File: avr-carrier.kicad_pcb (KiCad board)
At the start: 2 copper layers, 71.5 x 71.5 mm, 0 parts

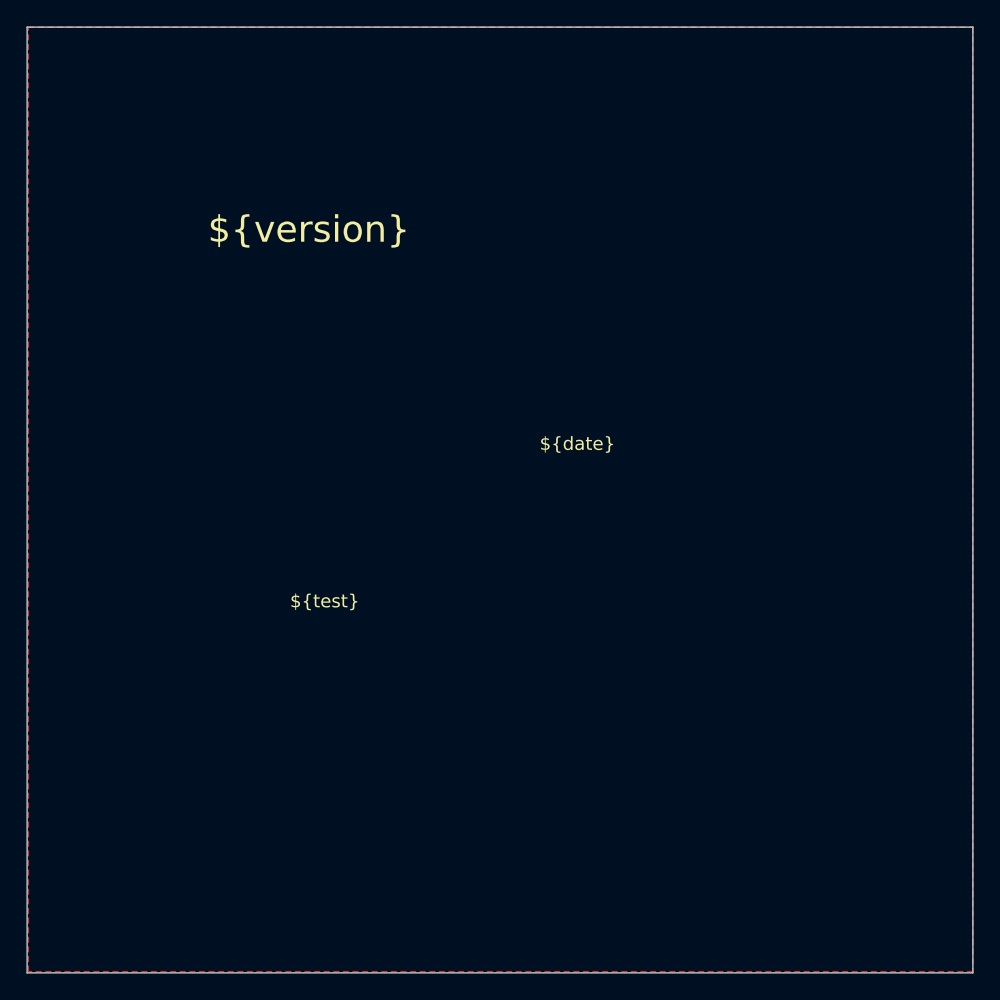
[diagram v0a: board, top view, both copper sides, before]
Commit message: init
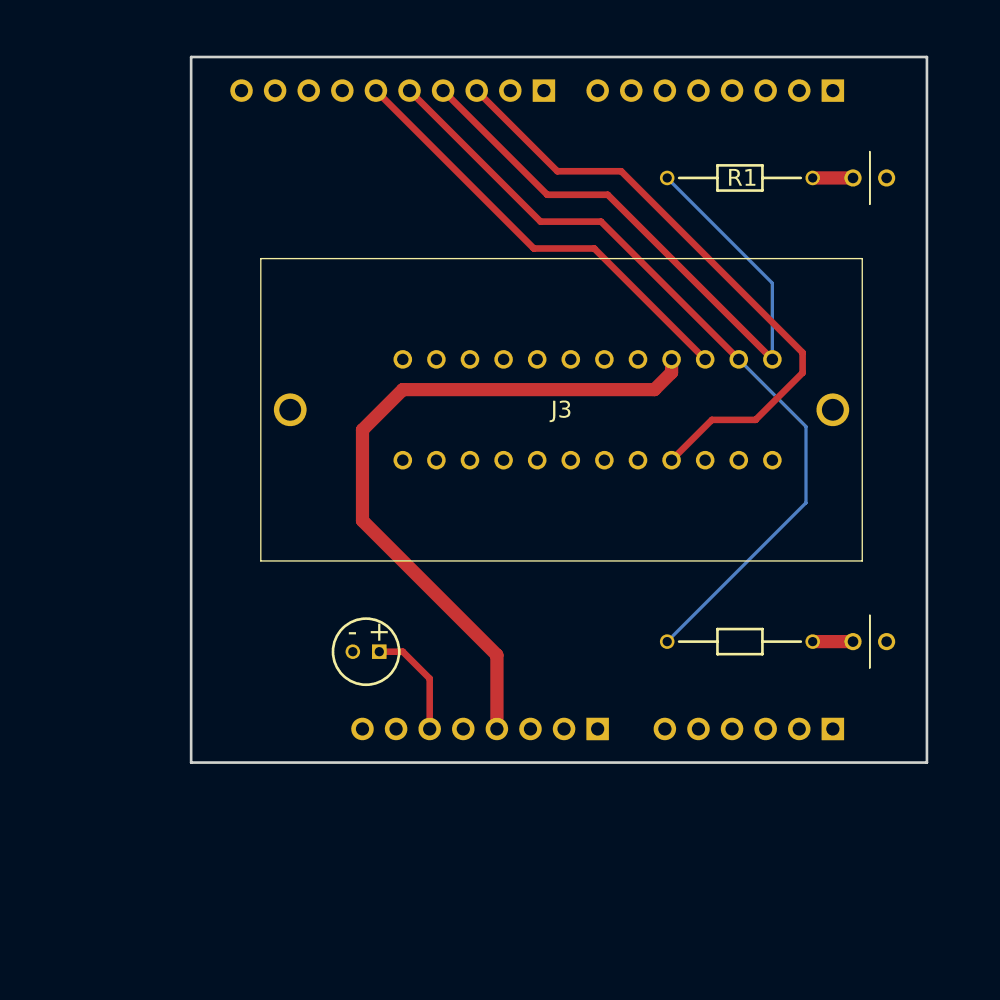
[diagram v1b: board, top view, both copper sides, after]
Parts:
- added C1: 860020372001, 860020372001:CAPPRD200W52D500H1250, F.Cu at (120.0, 117.0)
- added D1: LED, LTL-4232:LTL4232, F.Cu at (158.4, 81.2)
- added D2: LED, LTL-4232:LTL4232, F.Cu at (158.4, 116.3)
- added G***: LOGO, library:one, B.Cu at (135.0, 90.1)
- added J1: Conn_01x10, Connector_PinHeader_2.54mm:PinHeader_1x10_P2.54mm_Vertical, B.Cu at (132.5, 74.6)
- added J2: Conn_01x08, Connector_PinHeader_2.54mm:PinHeader_1x08_P2.54mm_Vertical, B.Cu at (136.5, 122.9)
- added J3: 24-3553-10, 24-3553-10:24355310, F.Cu at (121.8, 94.9)
- added J4: Conn_01x08, Connector_PinHeader_2.54mm:PinHeader_1x08_P2.54mm_Vertical, B.Cu at (154.3, 74.6)
- added J5: Conn_01x06, Connector_PinHeader_2.54mm:PinHeader_1x06_P2.54mm_Vertical, B.Cu at (154.3, 122.9)
- added R1: 100k, CFR-12JR-52-300R:RESAD1100W50L340D190, F.Cu at (152.8, 81.2)
- added R2: 100k, CFR-12JR-52-300R:RESAD1100W50L340D190, F.Cu at (152.8, 116.3)
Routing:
- net (no net): track 0.00 -> 259.3 mm
- added copper zone on B.Cu, net (none)
- removed copper zone on F.Cu, net (none)
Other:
- board size 71.5 x 71.5 mm -> 55.6 x 53.3 mm
- board text added: "+"
- board text added: "-"
- board text removed: "${date}"
- board text removed: "${test}"
- board text removed: "${version}"
